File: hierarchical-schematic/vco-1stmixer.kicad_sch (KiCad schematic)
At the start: 44 parts, among them J101 VCO Control In, J102 1st IF Out, J103 VCO Sample, J104 RF In, J105 Conn_01x02, U101 POS-200, U102 MAV-11, U103 MAV-11, U104 TUF-1H+

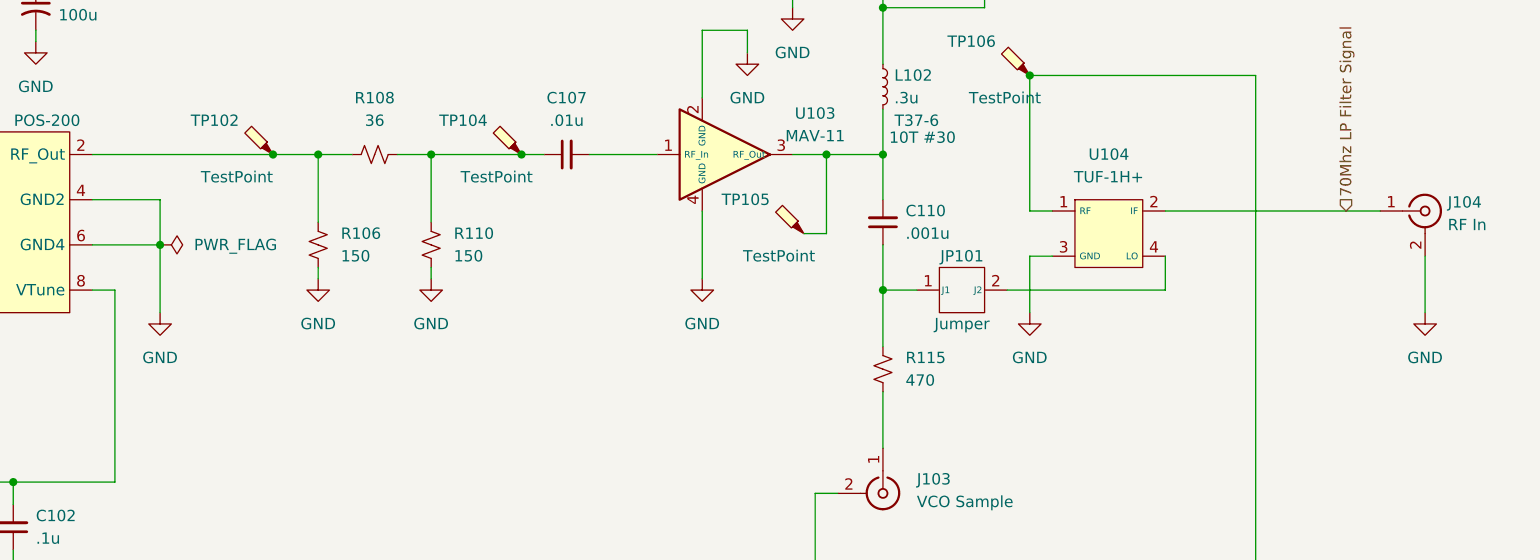
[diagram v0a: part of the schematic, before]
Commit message: hierarchical schematic updated to pass erc
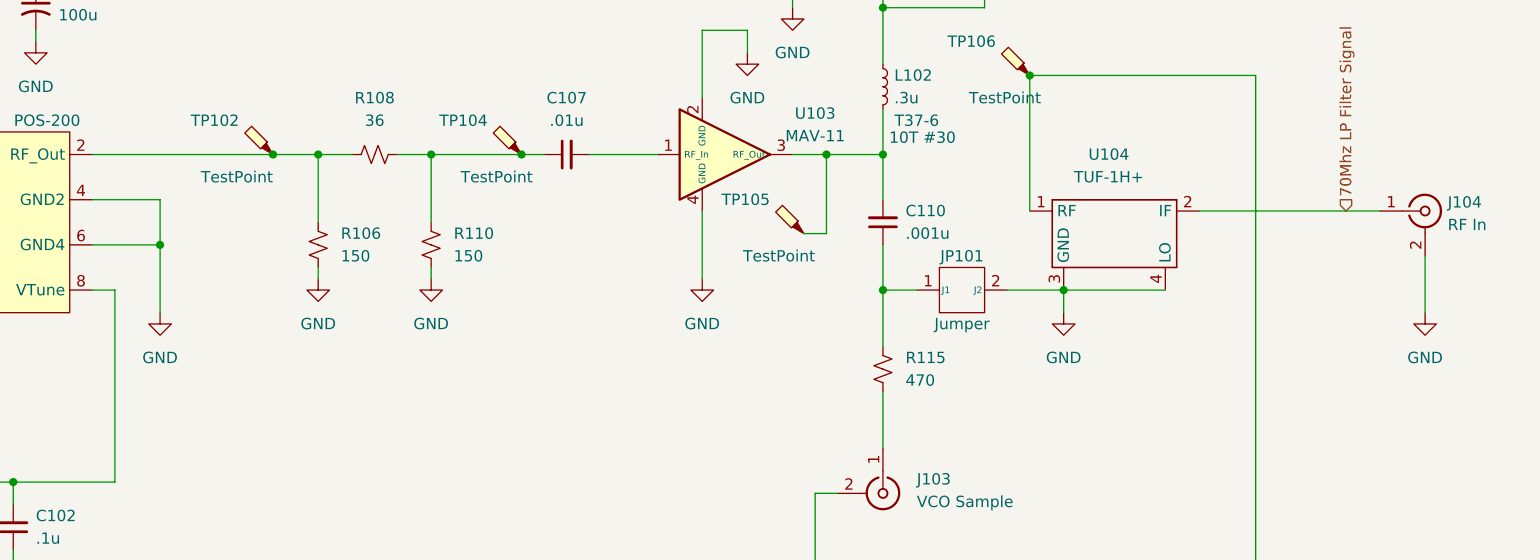
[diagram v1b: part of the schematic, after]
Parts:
- JP101: symbol vco-1stmixer:22284028 -> spectrum analyzer:22284028
- U101: symbol vco-1stmixer:POS-200 -> spectrum analyzer:POS-200
- U102, U103: symbol vco-1stmixer:MAV-11 -> spectrum analyzer:MAV-11
- U104: symbol vco-1stmixer:TUF-1H+ -> spectrum analyzer:TUF-1H+
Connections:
- net GND: now also JP101.2 (J2), U104.4 (LO)
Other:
- title: (none) -> Spectrum Analyzer: VCO 1st Mixer
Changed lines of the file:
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@@
   (paper "USLegal")
   (title_block
+    (title "Spectrum Analyzer: VCO 1st Mixer")
+    (date "2022-08-24")
+    (rev "0")
     (company "Andy McCann KA3KAF and Doug McCann KA3KAG")
     (comment 2 "Terry White K7TAU")
@@
   (junction (at 205.74 77.47) (diameter 0) (color 0 0 0 0)
   )
+  (junction (at 226.06 92.71) (diameter 0) (color 0 0 0 0)
+  )
   (junction (at 152.4 180.34) (diameter 0) (color 0 0 0 0)
   )
@@
     (stroke (width 0) (type default) (color 0 0 0 0))
   )
-  (wire (pts (xy 224.79 88.9) (xy 222.25 88.9))
-    (stroke (width 0) (type default) (color 0 0 0 0))
-  )
   (wire (pts (xy 85.09 187.96) (xy 85.09 180.34))
     (stroke (width 0) (type default) (color 0 0 0 0))
   )
+  (wire (pts (xy 226.06 92.71) (xy 237.49 92.71))
+    (stroke (width 0) (type default) (color 0 0 0 0))
+  )
   (wire (pts (xy 222.25 83.82) (xy 222.25 68.58))
     (stroke (width 0) (type default) (color 0 0 0 0))
@@
     (stroke (width 0) (type default) (color 0 0 0 0))
   )
-  (wire (pts (xy 224.79 83.82) (xy 222.25 83.82))
-    (stroke (width 0) (type default) (color 0 0 0 0))
-  )
   (wire (pts (xy 85.09 194.31) (xy 85.09 193.04))
     (stroke (width 0) (type default) (color 0 0 0 0))
@@
     (stroke (width 0) (type default) (color 0 0 0 0))
   )
-  (wire (pts (xy 237.49 92.71) (xy 219.71 92.71))
-    (stroke (width 0) (type default) (color 0 0 0 0))
-  )
   (wire (pts (xy 205.74 92.71) (xy 205.74 87.63))
     (stroke (width 0) (type default) (color 0 0 0 0))
@@
     (stroke (width 0) (type default) (color 0 0 0 0))
   )
-  (wire (pts (xy 261.62 83.82) (xy 237.49 83.82))
+  (wire (pts (xy 261.62 83.82) (xy 241.3 83.82))
     (stroke (width 0) (type default) (color 0 0 0 0))
   )
@@
     (stroke (width 0) (type default) (color 0 0 0 0))
   )
+  (wire (pts (xy 226.06 92.71) (xy 226.06 95.25))
+    (stroke (width 0) (type default) (color 0 0 0 0))
+  )
   (wire (pts (xy 142.24 149.86) (xy 142.24 153.67))
     (stroke (width 0) (type default) (color 0 0 0 0))
@@
     (stroke (width 0) (type default) (color 0 0 0 0))
   )
-  (wire (pts (xy 237.49 88.9) (xy 237.49 92.71))
-    (stroke (width 0) (type default) (color 0 0 0 0))
-  )
   (wire (pts (xy 85.09 140.97) (xy 85.09 180.34))
     (stroke (width 0) (type default) (color 0 0 0 0))
@@
     (stroke (width 0) (type default) (color 0 0 0 0))
   )
+  (wire (pts (xy 219.71 92.71) (xy 226.06 92.71))
+    (stroke (width 0) (type default) (color 0 0 0 0))
+  )
   (wire (pts (xy 199.39 86.36) (xy 199.39 77.47))
     (stroke (width 0) (type default) (color 0 0 0 0))
@@
   )
   (wire (pts (xy 160.02 149.86) (xy 152.4 149.86))
-    (stroke (width 0) (type default) (color 0 0 0 0))
-  )
-  (wire (pts (xy 222.25 88.9) (xy 222.25 95.25))
     (stroke (width 0) (type default) (color 0 0 0 0))
   )
@@
     (effects (font (size 1.27 1.27)) (justify right))
   )
-  (symbol (lib_id "vco-1stmixer:TUF-1H+") (at 231.14 86.36 0) (unit 1)
+  (symbol (lib_id "spectrum analyzer:TUF-1H+") (at 231.14 86.36 0) (unit 1)
     (in_bom yes) (on_board yes)
     (property "Reference" "U104" (id 0) (at 231.14 77.47 0))
     (property "Value" "TUF-1H+" (id 1) (at 231.14 80.01 0))
-    (property "Footprint" "vco-1stmixer:TUF-1H" (id 2) (at 218.44 96.52 0)
-      (effects (font (size 1.27 1.27)) hide)
-    )
-    (property "Datasheet" "https://www.minicircuits.com/pdfs/TUF-1H+.pdf" (id 3) (at 231.14 93.98 0)
+    (property "Footprint" "vco-1stmixer:TUF-1H" (id 2) (at 231.14 86.36 0)
+      (effects (font (size 1.27 1.27)) hide)
+    )
+    (property "Datasheet" "https://www.minicircuits.com/pdfs/TUF-1H+.pdf" (id 3) (at 231.14 86.36 0)
       (effects (font (size 1.27 1.27)) hide)
     )
@@
     (pin "2")
   )
-  (symbol (lib_id "vco-1stmixer:22284028") (at 214.63 92.71 0) (unit 1)
+  (symbol (lib_id "spectrum analyzer:22284028") (at 214.63 92.71 0) (unit 1)
     (in_bom yes) (on_board yes)
     (property "Reference" "JP101" (id 0) (at 214.63 88.9 0))
     (property "Value" "Jumper" (id 1) (at 214.63 96.52 0))
-    (property "Footprint" "vco-1stmixer:22284028" (id 2) (at 214.63 86.614 0)
+    (property "Footprint" "vco-1stmixer:22284028" (id 2) (at 215.9 96.52 0)
       (effects (font (size 1.524 1.524)) hide)
     )
@@
     (pin "1")
   )
-  (symbol (lib_id "vco-1stmixer:MAV-11") (at 185.42 77.47 0) (unit 1)
+  (symbol (lib_id "spectrum analyzer:MAV-11") (at 185.42 77.47 0) (unit 1)
     (in_bom yes) (on_board yes) (fields_autoplaced)
     (property "Reference" "U103" (id 0) (at 198.12 72.8533 0))
@@
     (pin "2")
   )
-  (symbol (lib_name "MAV-11_1") (lib_id "vco-1stmixer:MAV-11") (at 130.81 180.34 0) (unit 1)
+  (symbol (lib_id "spectrum analyzer:MAV-11") (at 130.81 180.34 0) (unit 1)
     (in_bom yes) (on_board yes) (fields_autoplaced)
     (property "Reference" "U102" (id 0) (at 143.51 175.7233 0))
@@
     (pin "2")
   )
-  (symbol (lib_id "power:PWR_FLAG") (at 124.46 87.63 270) (unit 1)
-    (in_bom yes) (on_board yes) (fields_autoplaced)
-    (property "Reference" "#FLG0102" (id 0) (at 126.365 87.63 0)
-      (effects (font (size 1.27 1.27)) hide)
-    )
-    (property "Value" "PWR_FLAG" (id 1) (at 128.27 87.6299 90)
-      (effects (font (size 1.27 1.27)) (justify left))
-    )
-    (property "Footprint" "" (id 2) (at 124.46 87.63 0)
-      (effects (font (size 1.27 1.27)) hide)
-    )
-    (property "Datasheet" "~" (id 3) (at 124.46 87.63 0)
-      (effects (font (size 1.27 1.27)) hide)
-    )
-    (pin "1")
-  )
   (symbol (lib_id "Connector:Conn_Coaxial") (at 205.74 115.57 270) (unit 1)
     (in_bom yes) (on_board yes) (fields_autoplaced)
@@
     (pin "2")
   )
-  (symbol (lib_id "vco-1stmixer:POS-200") (at 106.68 85.09 0) (unit 1)
+  (symbol (lib_id "spectrum analyzer:POS-200") (at 106.68 85.09 0) (unit 1)
     (in_bom yes) (on_board yes)
     (property "Reference" "U101" (id 0) (at 99.06 73.66 0))
     (property "Value" "POS-200" (id 1) (at 111.76 73.66 0))
-    (property "Footprint" "vco-1stmixer:POS-200" (id 2) (at 106.68 82.55 0)
-      (effects (font (size 1.27 1.27)) hide)
-    )
-    (property "Datasheet" "" (id 3) (at 106.68 82.55 0)
+    (property "Footprint" "vco-1stmixer:POS-200" (id 2) (at 106.68 97.79 0)
+      (effects (font (size 1.27 1.27)) hide)
+    )
+    (property "Datasheet" "https://www.mini-circuits.com/pdfs/POS-200+.pdf" (id 3) (at 106.68 96.52 0)
       (effects (font (size 1.27 1.27)) hide)
     )
@@
     (pin "1")
   )
-  (symbol (lib_id "power:GND") (at 222.25 95.25 0) (unit 1)
-    (in_bom yes) (on_board yes) (fields_autoplaced)
-    (property "Reference" "#PWR0120" (id 0) (at 222.25 101.6 0)
-      (effects (font (size 1.27 1.27)) hide)
-    )
-    (property "Value" "GND" (id 1) (at 222.25 100.33 0))
-    (property "Footprint" "" (id 2) (at 222.25 95.25 0)
-      (effects (font (size 1.27 1.27)) hide)
-    )
-    (property "Datasheet" "" (id 3) (at 222.25 95.25 0)
-      (effects (font (size 1.27 1.27)) hide)
-    )
+  (symbol (lib_id "power:GND") (at 226.06 95.25 0) (unit 1)
+    (in_bom yes) (on_board yes) (fields_autoplaced)
+    (property "Reference" "#PWR0120" (id 0) (at 226.06 101.6 0)
+      (effects (font (size 1.27 1.27)) hide)
+    )
+    (property "Value" "GND" (id 1) (at 226.06 100.33 0))
+    (property "Footprint" "" (id 2) (at 226.06 95.25 0)
+      (effects (font (size 1.27 1.27)) hide)
+    )
+    (property "Datasheet" "" (id 3) (at 226.06 95.25 0)
+      (effects (font (size 1.27 1.27)) hide)
+    )

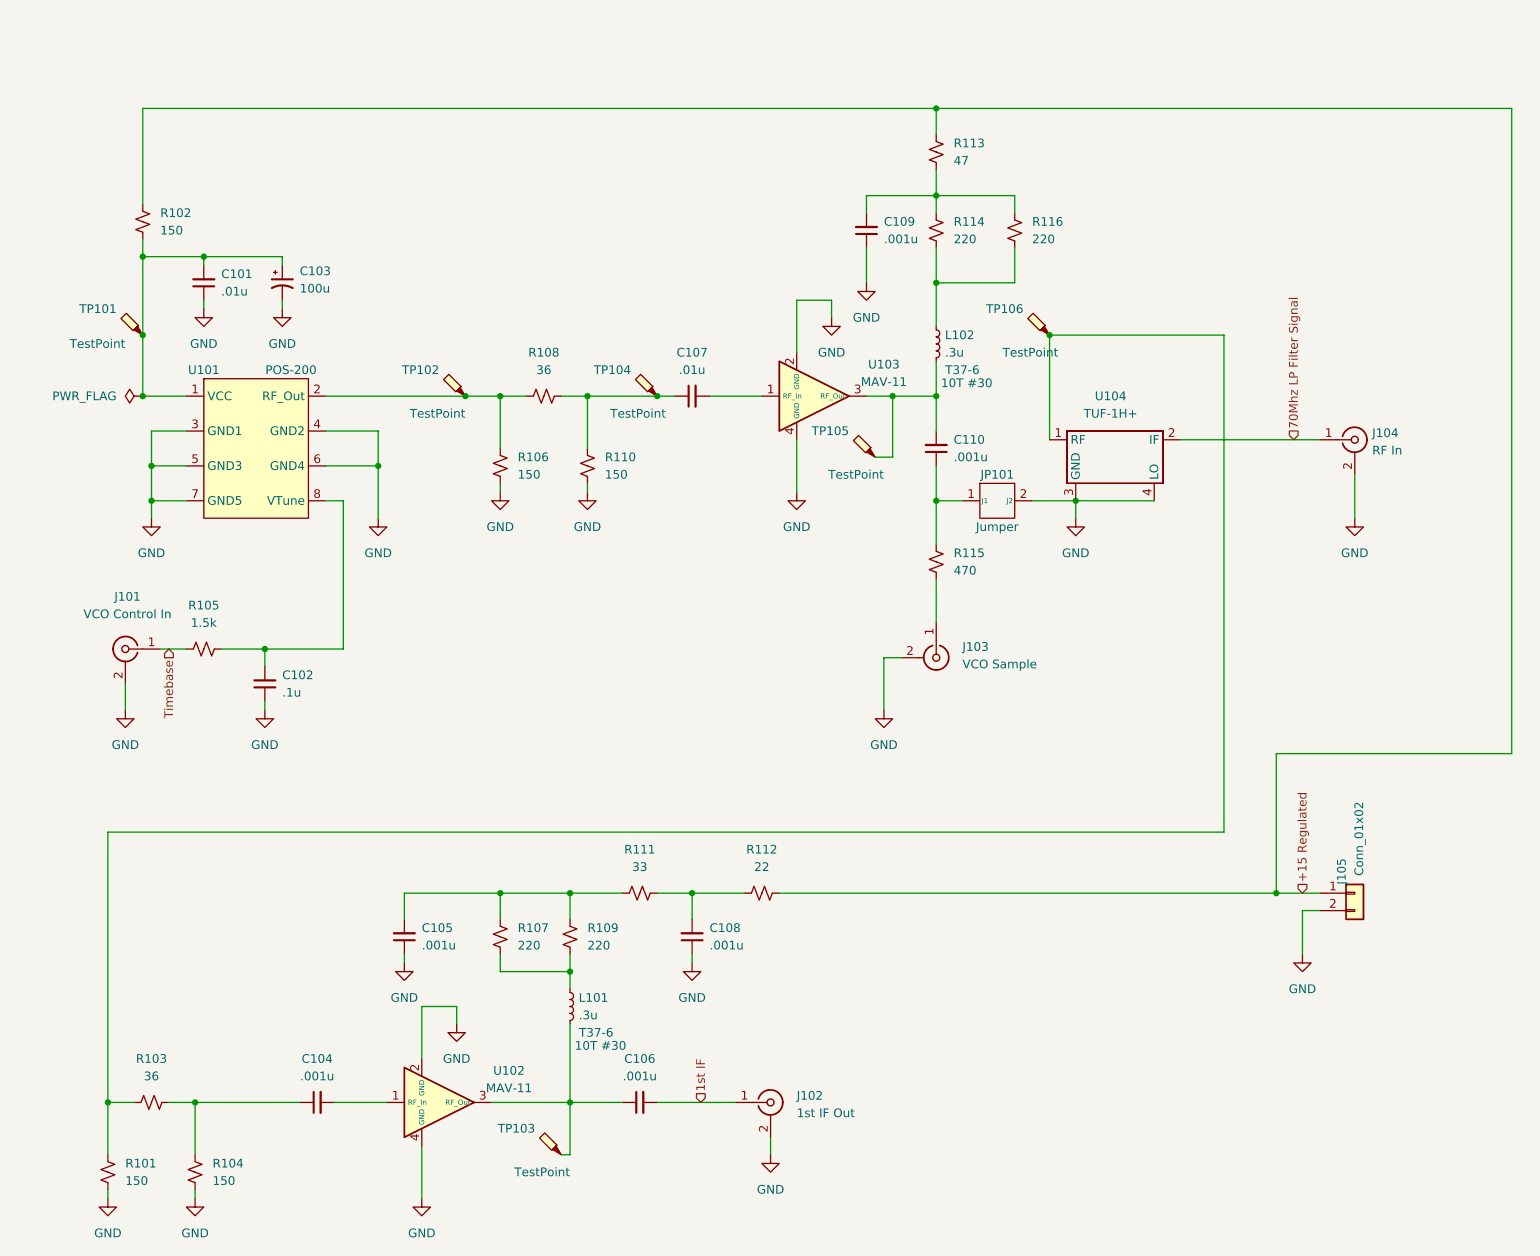
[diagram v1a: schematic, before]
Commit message: appearance improvements
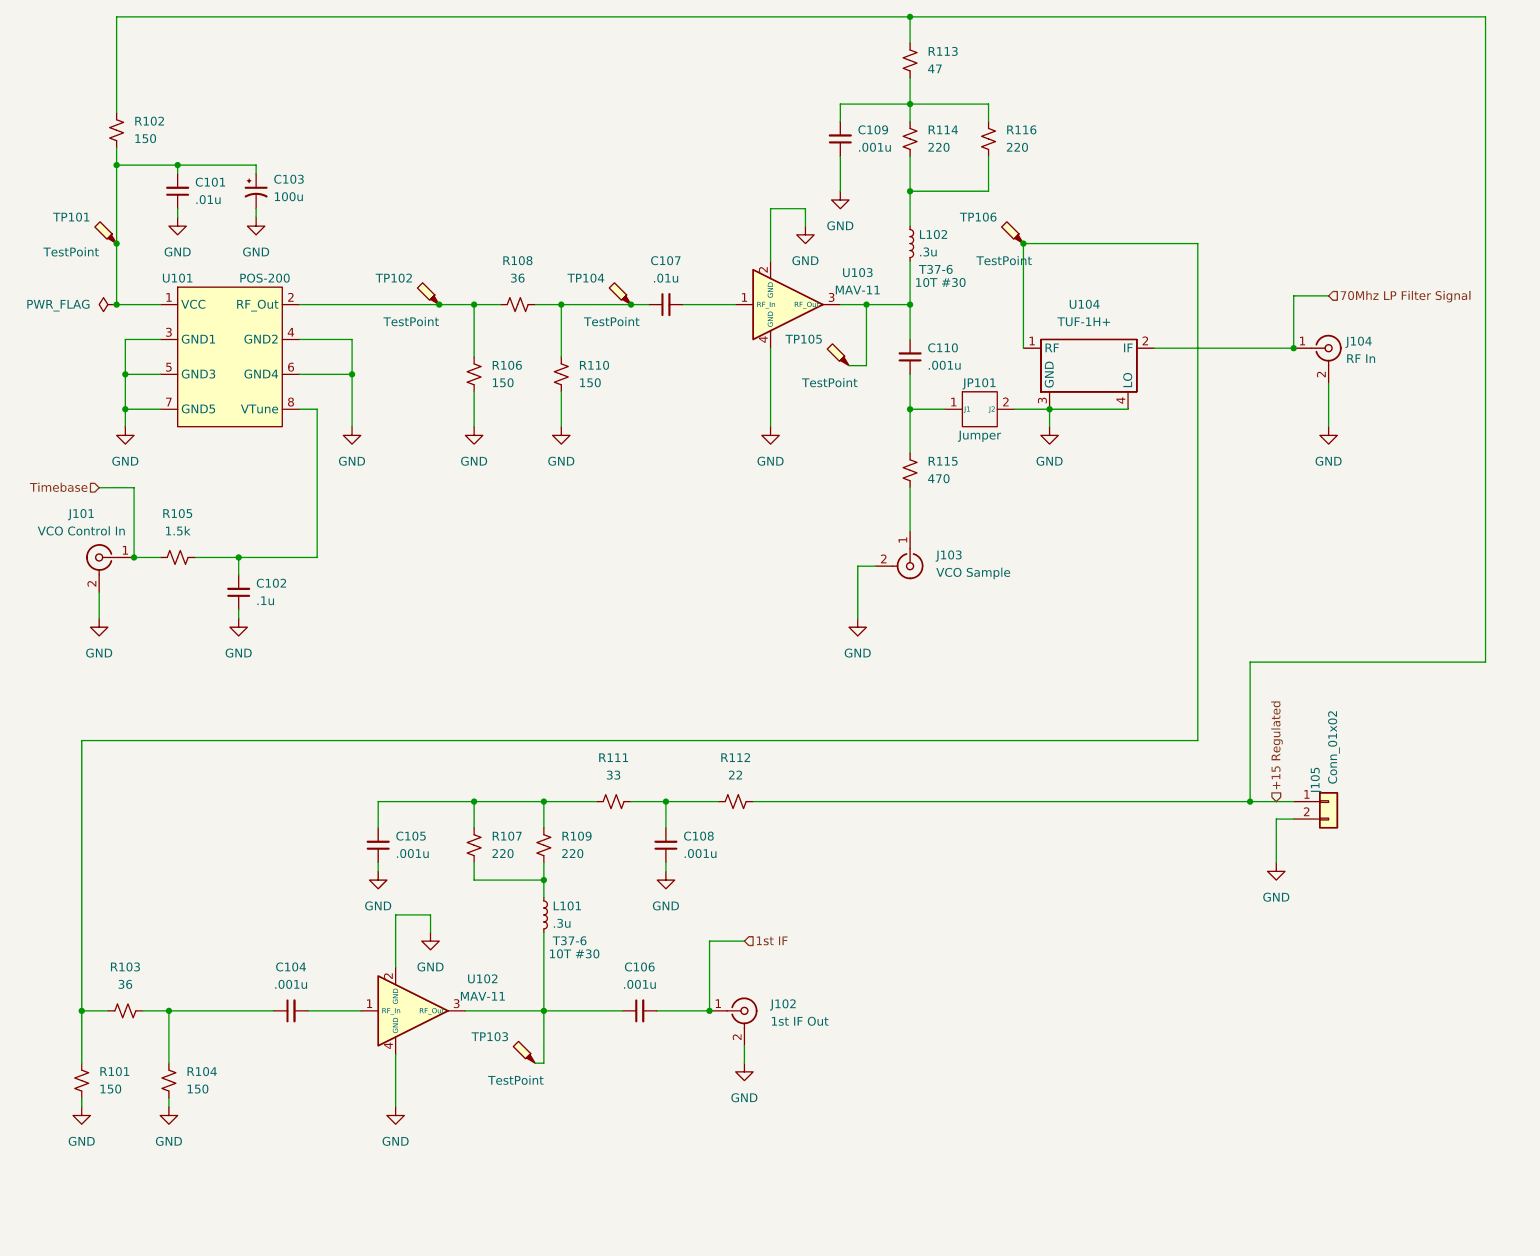
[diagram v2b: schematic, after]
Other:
- moved on the sheet: C101, C102, C103, C104, C105, C106, C107, C108, C109, C110, J101, J102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
